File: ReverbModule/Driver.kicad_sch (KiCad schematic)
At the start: 29 parts, among them J1 Tank, J2 Screw_Terminal_01x02, Q1 BD139, Q2 BD140, U1 NE5532

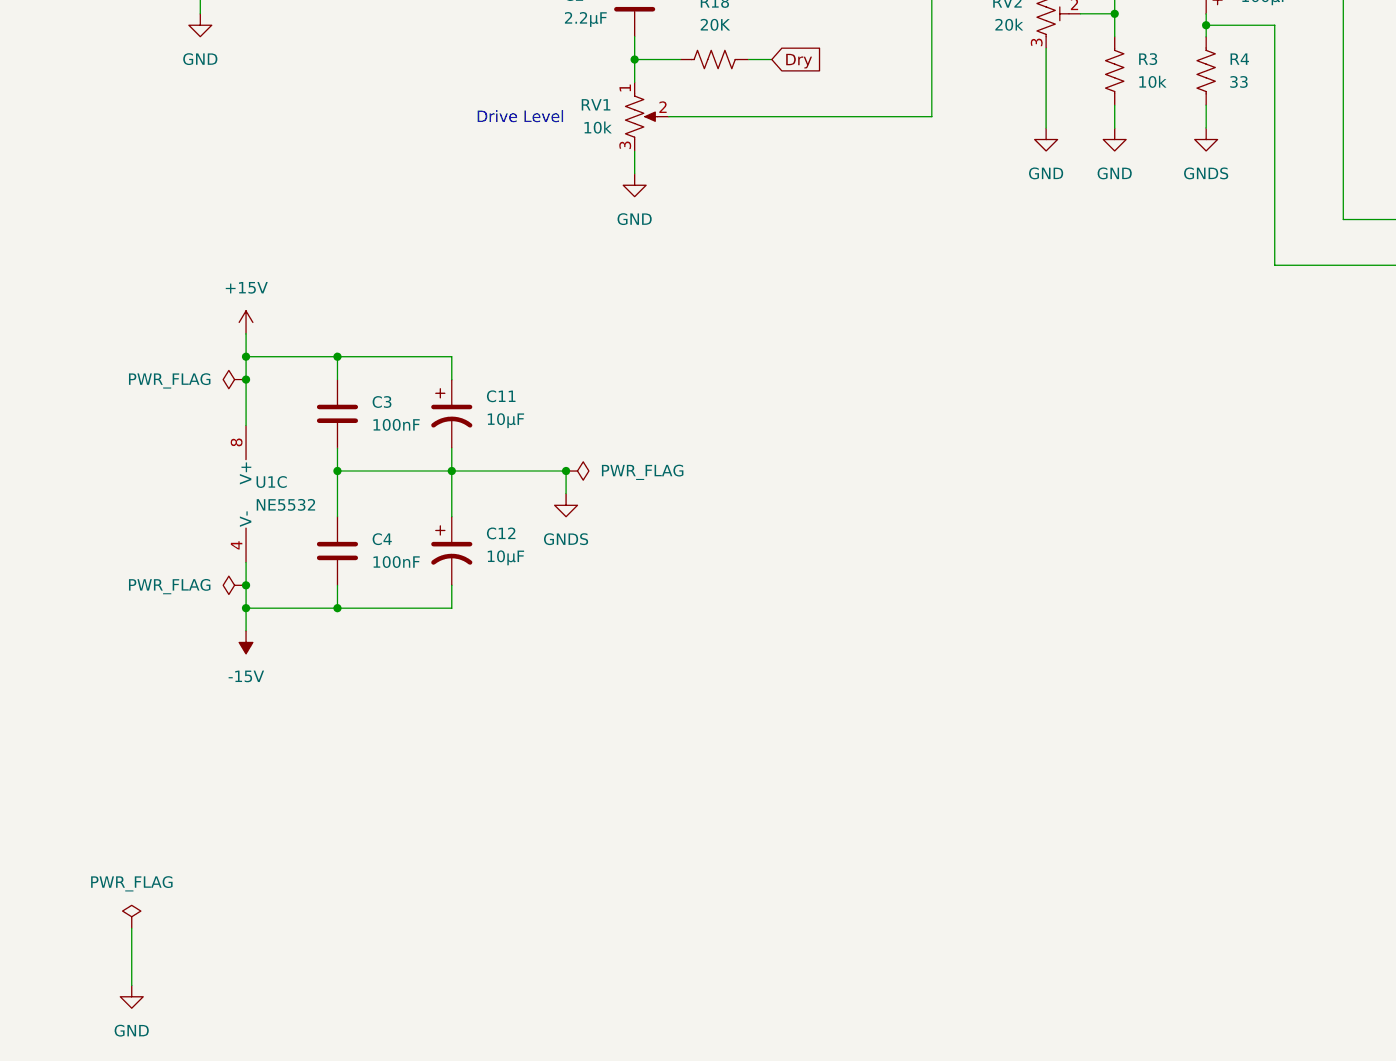
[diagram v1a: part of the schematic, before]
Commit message: Capture Complete
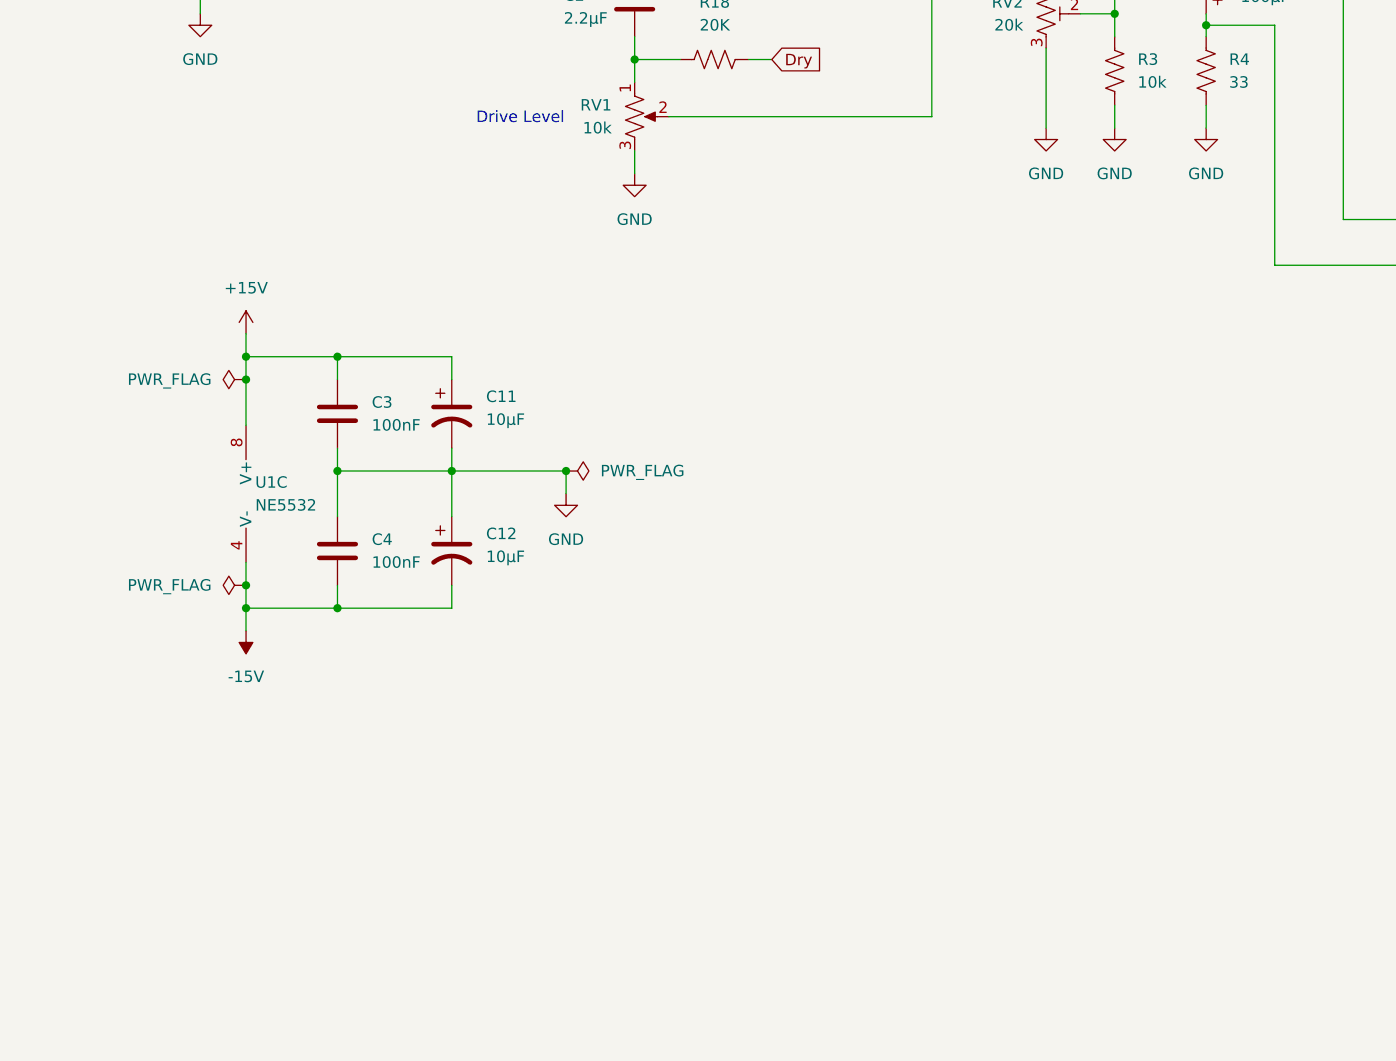
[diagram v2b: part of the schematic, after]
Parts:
- C8: footprint (none) -> Capacitor_THT:CP_Radial_D8.0mm_P3.50mm; MPN (none) -> UPW1H101MPD
- J1: footprint (none) -> TerminalBlock_Phoenix:TerminalBlock_Phoenix_MKDS-1,5-2-5.08_1x02_P5.08mm_Horizontal
- R18: footprint (none) -> Resistor_SMD:R_0805_2012Metric_Pad1.20x1.40mm_HandSolder; LCSC (none) -> C4328; MPN (none) -> 0805W8F2002T5E
- RV1, RV2: footprint (none) -> TerminalBlock_Phoenix:TerminalBlock_Phoenix_MKDS-1,5-3-5.08_1x03_P5.08mm_Horizontal
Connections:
- net GNDS is gone; now on net GND: C11.2, C12.1, C3.2, C4.1, R4.2
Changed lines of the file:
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@@
 	(wire
 		(pts
-			(xy 25.4 177.8) (xy 25.4 184.15)
-		)
-		(stroke
-			(width 0)
-			(type default)
-		)
-	)
-	(wire
-		(pts
 			(xy 203.2 38.1) (xy 220.98 38.1)
 		)
@@
 	)
 	(symbol
-		(lib_id "power:GND")
-		(at 25.4 184.15 0)
-		(unit 1)
-		(body_style 1)
-		(exclude_from_sim no)
-		(in_bom yes)
-		(on_board yes)
-		(in_pos_files yes)
-		(dnp no)
-		(fields_autoplaced yes)
-		(property "Reference" "#PWR04"
-			(at 25.4 190.5 0)
-			(hide yes)
-			(show_name no)
-			(do_not_autoplace no)
-			(effects
-				(font
-					(size 1.27 1.27)
-				)
-			)
-		)
-		(property "Value" "GND"
-			(at 25.4 189.23 0)
-			(show_name no)
-			(do_not_autoplace no)
-			(effects
-				(font
-					(size 1.27 1.27)
-				)
-			)
-		)
-		(property "Footprint" ""
-			(at 25.4 184.15 0)
-			(hide yes)
-			(show_name no)
-			(do_not_autoplace no)
-			(effects
-				(font
-					(size 1.27 1.27)
-				)
-			)
-		)
-		(property "Datasheet" ""
-			(at 25.4 184.15 0)
-			(hide yes)
-			(show_name no)
-			(do_not_autoplace no)
-			(effects
-				(font
-					(size 1.27 1.27)
-				)
-			)
-		)
-		(property "Description" "Power symbol creates a global label with name \"GND\" , ground"
-			(at 25.4 184.15 0)
-			(hide yes)
-			(show_name no)
-			(do_not_autoplace no)
-			(effects
-				(font
-					(size 1.27 1.27)
-				)
-			)
-		)
-		(pin "1"
-		)
-		(instances
-			(project "ReverbModule"
-				(path "/e19e1d15-f0b3-4286-a818-bc907405212b/c6d45d4c-e85e-4a36-afcc-7c11e84777bd"
-					(reference "#PWR04")
-					(unit 1)
-				)
-			)
-		)
-	)
-	(symbol
 		(lib_id "Device:C_Polarized_US")
 		(at 200.66 69.85 0)
@@
 	)
 	(symbol
+		(lib_id "power:GND")
+		(at 144.78 88.9 0)
+		(unit 1)
+		(body_style 1)
+		(exclude_from_sim no)
+		(in_bom yes)
+		(on_board yes)
+		(in_pos_files yes)
+		(dnp no)
+		(fields_autoplaced yes)
+		(property "Reference" "#PWR05"
+			(at 144.78 95.25 0)
+			(hide yes)
+			(show_name no)
+			(do_not_autoplace no)
+			(effects
+				(font
+					(size 1.27 1.27)
+				)
+			)
+		)
+		(property "Value" "GND"
+			(at 144.78 93.98 0)
+			(show_name no)
+			(do_not_autoplace no)
+			(effects
+				(font
+					(size 1.27 1.27)
+				)
+			)
+		)
+		(property "Footprint" ""
+			(at 144.78 88.9 0)
+			(hide yes)
+			(show_name no)
+			(do_not_autoplace no)
+			(effects
+				(font
+					(size 1.27 1.27)
+				)
+			)
+		)
+		(property "Datasheet" ""
+			(at 144.78 88.9 0)
+			(hide yes)
+			(show_name no)
+			(do_not_autoplace no)
+			(effects
+				(font
+					(size 1.27 1.27)
+				)
+			)
+		)
+		(property "Description" "Power symbol creates a global label with name \"GND\" , ground"
+			(at 144.78 88.9 0)
+			(hide yes)
+			(show_name no)
+			(do_not_autoplace no)
+			(effects
+				(font
+					(size 1.27 1.27)
+				)
+			)
+		)
+		(pin "1"
+		)
+		(instances
+			(project "ReverbModule"
+				(path "/e19e1d15-f0b3-4286-a818-bc907405212b/c6d45d4c-e85e-4a36-afcc-7c11e84777bd"
+					(reference "#PWR05")
+					(unit 1)
+				)
+			)
+		)
+	)
+	(symbol
 		(lib_id "Device:R_US")
 		(at 144.78 82.55 0)
@@
 	)
 	(symbol
-		(lib_id "power:GNDS")
-		(at 73.66 129.54 0)
-		(unit 1)
-		(body_style 1)
-		(exclude_from_sim no)
-		(in_bom yes)
-		(on_board yes)
-		(in_pos_files yes)
-		(dnp no)
-		(fields_autoplaced yes)
-		(property "Reference" "#PWR05"
-			(at 73.66 135.89 0)
-			(hide yes)
-			(show_name no)
-			(do_not_autoplace no)
-			(effects
-				(font
-					(size 1.27 1.27)
-				)
-			)
-		)
-		(property "Value" "GNDS"
-			(at 73.66 134.62 0)
-			(show_name no)
-			(do_not_autoplace no)
-			(effects
-				(font
-					(size 1.27 1.27)
-				)
-			)
-		)
-		(property "Footprint" ""
-			(at 73.66 129.54 0)
-			(hide yes)
-			(show_name no)
-			(do_not_autoplace no)
-			(effects
-				(font
-					(size 1.27 1.27)
-				)
-			)
-		)
-		(property "Datasheet" ""
-			(at 73.66 129.54 0)
-			(hide yes)
-			(show_name no)
-			(do_not_autoplace no)
-			(effects
-				(font
-					(size 1.27 1.27)
-				)
-			)
-		)
-		(property "Description" "Power symbol creates a global label with name \"GNDS\" , signal ground"
-			(at 73.66 129.54 0)
-			(hide yes)
-			(show_name no)
-			(do_not_autoplace no)
-			(effects
-				(font
-					(size 1.27 1.27)
-				)
-			)
-		)
-		(pin "1"
-		)
-		(instances
-			(project "ReverbModule"
-				(path "/e19e1d15-f0b3-4286-a818-bc907405212b/c6d45d4c-e85e-4a36-afcc-7c11e84777bd"
-					(reference "#PWR05")
-					(unit 1)
-				)
-			)
-		)
-	)
-	(symbol
 		(lib_id "Device:R_US")
 		(at 220.98 59.69 0)
@@
 			)
 		)
-		(property "Footprint" ""
+		(property "Footprint" "Capacitor_THT:CP_Radial_D8.0mm_P3.50mm"
 			(at 144.78 72.39 0)
 			(hide yes)
@@
 			)
 		)
-		(property "Description" "Polarized capacitor, US symbol"
+		(property "Description" "Nichicon UPW"
+			(at 144.78 72.39 0)
+			(hide yes)
+			(show_name no)
+			(do_not_autoplace no)
+			(effects
+				(font
+					(size 1.27 1.27)
+				)
+			)
+		)
+		(property "MPN" "UPW1H101MPD"
 			(at 144.78 72.39 0)
 			(hide yes)
@@
 	)
 	(symbol
-		(lib_id "power:GNDS")
-		(at 144.78 88.9 0)
+		(lib_id "power:GND")
+		(at 73.66 129.54 0)
 		(unit 1)
 		(body_style 1)
@@
 		(fields_autoplaced yes)
 		(property "Reference" "#PWR010"
-			(at 144.78 95.25 0)
+			(at 73.66 135.89 0)
 			(hide yes)
 			(show_name no)
@@
 			)
 		)
-		(property "Value" "GNDS"
-			(at 144.78 93.98 0)
+		(property "Value" "GND"
+			(at 73.66 134.62 0)
 			(show_name no)
 			(do_not_autoplace no)
@@
 		)
 		(property "Footprint" ""
-			(at 144.78 88.9 0)
+			(at 73.66 129.54 0)
 			(hide yes)
 			(show_name no)
@@
 		)
 		(property "Datasheet" ""
-			(at 144.78 88.9 0)
+			(at 73.66 129.54 0)
 			(hide yes)
 			(show_name no)
@@
 			)
 		)
-		(property "Description" "Power symbol creates a global label with name \"GNDS\" , signal ground"
-			(at 144.78 88.9 0)
+		(property "Description" "Power symbol creates a global label with name \"GND\" , ground"
+			(at 73.66 129.54 0)
 			(hide yes)
 			(show_name no)
@@
 			)
 		)
-		(property "Footprint" ""
+		(property "Footprint" "Resistor_SMD:R_0805_2012Metric_Pad1.20x1.40mm_HandSolder"
 			(at 90.424 80.264 90)
 			(hide yes)
@@
 			)
 		)
+		(property "MPN" "0805W8F2002T5E"
+			(at 90.17 81.28 90)
+			(hide yes)
+			(show_name no)
+			(do_not_autoplace no)
+			(effects
+				(font
+					(size 1.27 1.27)
+				)
+			)
+		)
+		(property "LCSC" "C4328"
+			(at 90.17 81.28 90)
+			(hide yes)
+			(show_name no)
+			(do_not_autoplace no)
+			(effects
+				(font
+					(size 1.27 1.27)
+				)
+			)
+		)
 		(pin "1"
 		)
@@
 	)
 	(symbol
-		(lib_id "power:PWR_FLAG")
-		(at 25.4 177.8 0)
-		(unit 1)
-		(body_style 1)
-		(exclude_from_sim no)
-		(in_bom yes)
-		(on_board yes)
-		(in_pos_files yes)
-		(dnp no)
-		(fields_autoplaced yes)
-		(property "Reference" "#FLG01"
-			(at 25.4 175.895 0)
-			(hide yes)
-			(show_name no)
-			(do_not_autoplace no)
-			(effects
-				(font
-					(size 1.27 1.27)
-				)
-			)
-		)
-		(property "Value" "PWR_FLAG"
-			(at 25.4 172.72 0)
-			(show_name no)
-			(do_not_autoplace no)
-			(effects
-				(font
-					(size 1.27 1.27)
-				)
-			)
-		)
-		(property "Footprint" ""
-			(at 25.4 177.8 0)
-			(hide yes)
-			(show_name no)
-			(do_not_autoplace no)
-			(effects
-				(font
-					(size 1.27 1.27)
-				)
-			)
-		)
-		(property "Datasheet" ""
-			(at 25.4 177.8 0)
-			(hide yes)
-			(show_name no)
-			(do_not_autoplace no)
-			(effects
-				(font
-					(size 1.27 1.27)
-				)
-			)
-		)
-		(property "Description" "Special symbol for telling ERC where power comes from"
-			(at 25.4 177.8 0)
-			(hide yes)
-			(show_name no)
-			(do_not_autoplace no)
-			(effects
-				(font
-					(size 1.27 1.27)
-				)
-			)
-		)
-		(pin "1"
-		)
-		(instances
-			(project "ReverbModule"
-				(path "/e19e1d15-f0b3-4286-a818-bc907405212b/c6d45d4c-e85e-4a36-afcc-7c11e84777bd"
-					(reference "#FLG01")
-					(unit 1)
-				)
-			)
-		)
-	)
-	(symbol
 		(lib_id "power:+15V")
 		(at 203.2 35.56 0)
@@
 			)
 		)
-		(property "Footprint" ""
+		(property "Footprint" "TerminalBlock_Phoenix:TerminalBlock_Phoenix_MKDS-1,5-3-5.08_1x03_P5.08mm_Horizontal"
 			(at 81.28 87.63 0)
 			(hide yes)
@@
 			)
 		)
-		(property "Footprint" ""
+		(property "Footprint" "TerminalBlock_Phoenix:TerminalBlock_Phoenix_MKDS-1,5-3-5.08_1x03_P5.08mm_Horizontal"
 			(at 127 76.2 0)
 			(hide yes)
@@
 			)
 		)
-		(property "Footprint" ""
+		(property "Footprint" "TerminalBlock_Phoenix:TerminalBlock_Phoenix_MKDS-1,5-2-5.08_1x02_P5.08mm_Horizontal"
 			(at 238.76 63.5 0)
 			(hide yes)
